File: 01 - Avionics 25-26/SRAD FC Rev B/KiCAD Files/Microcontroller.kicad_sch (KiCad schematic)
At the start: 4 parts

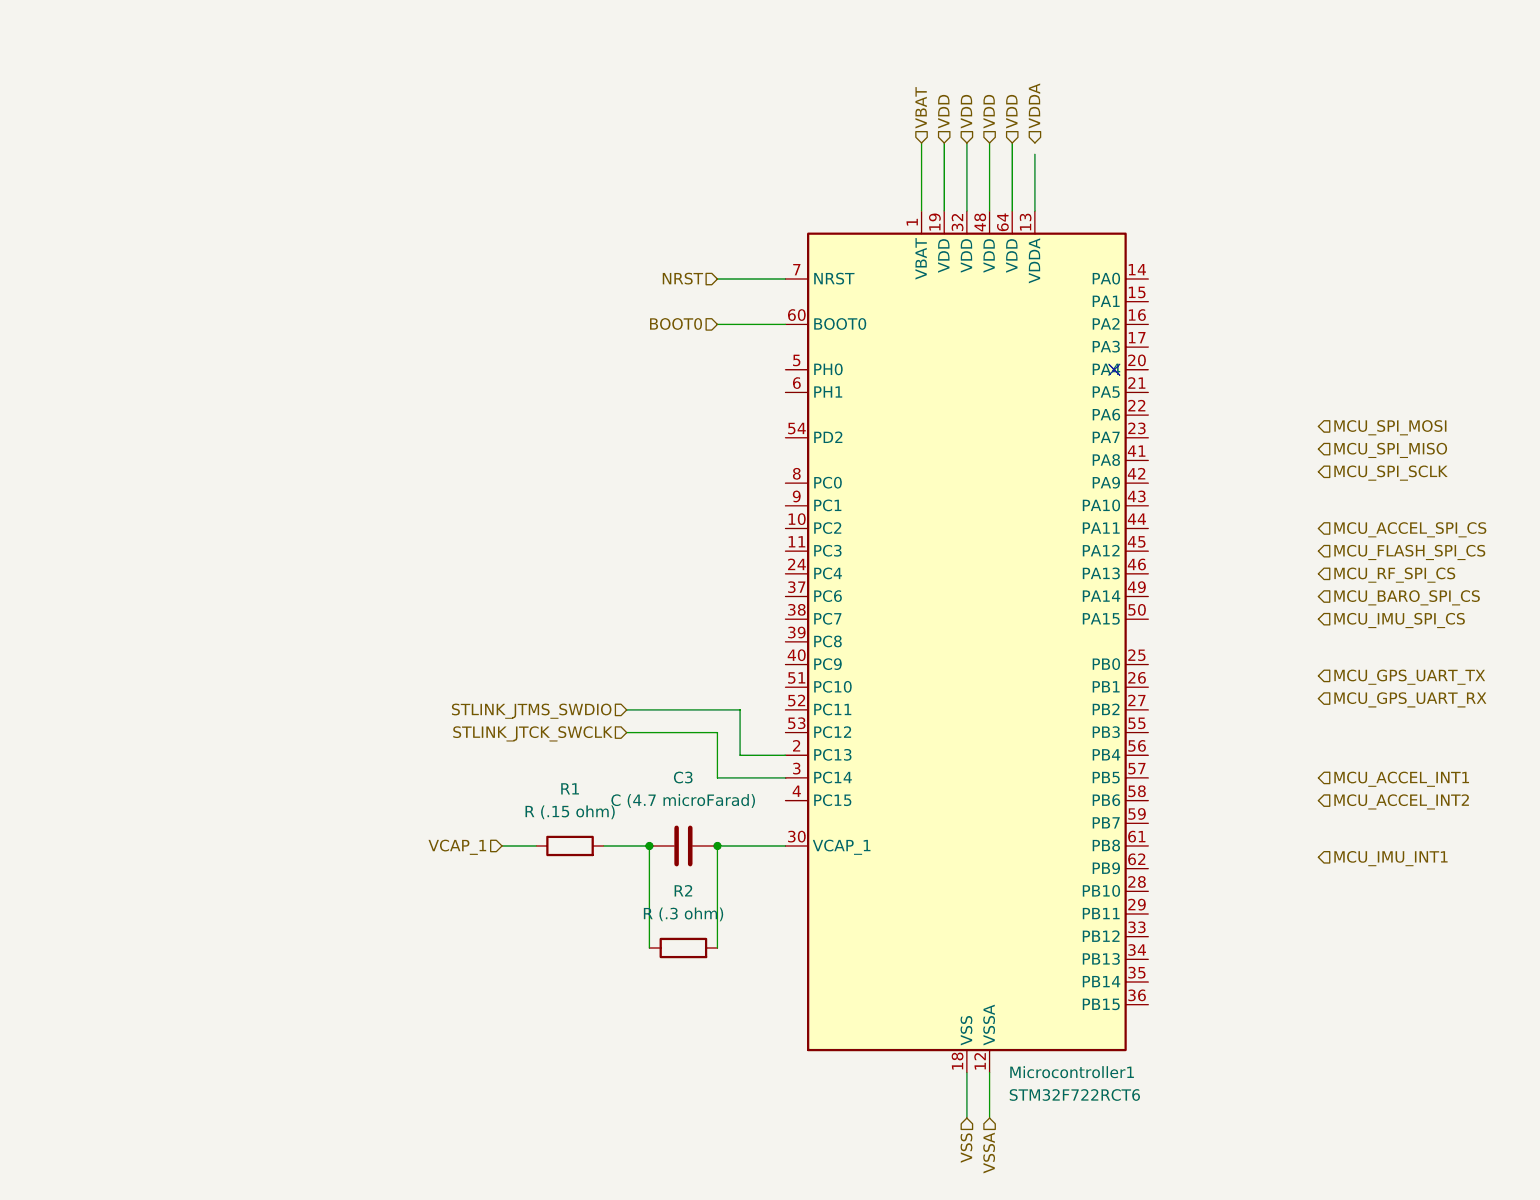
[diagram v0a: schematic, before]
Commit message: moved..... stuff
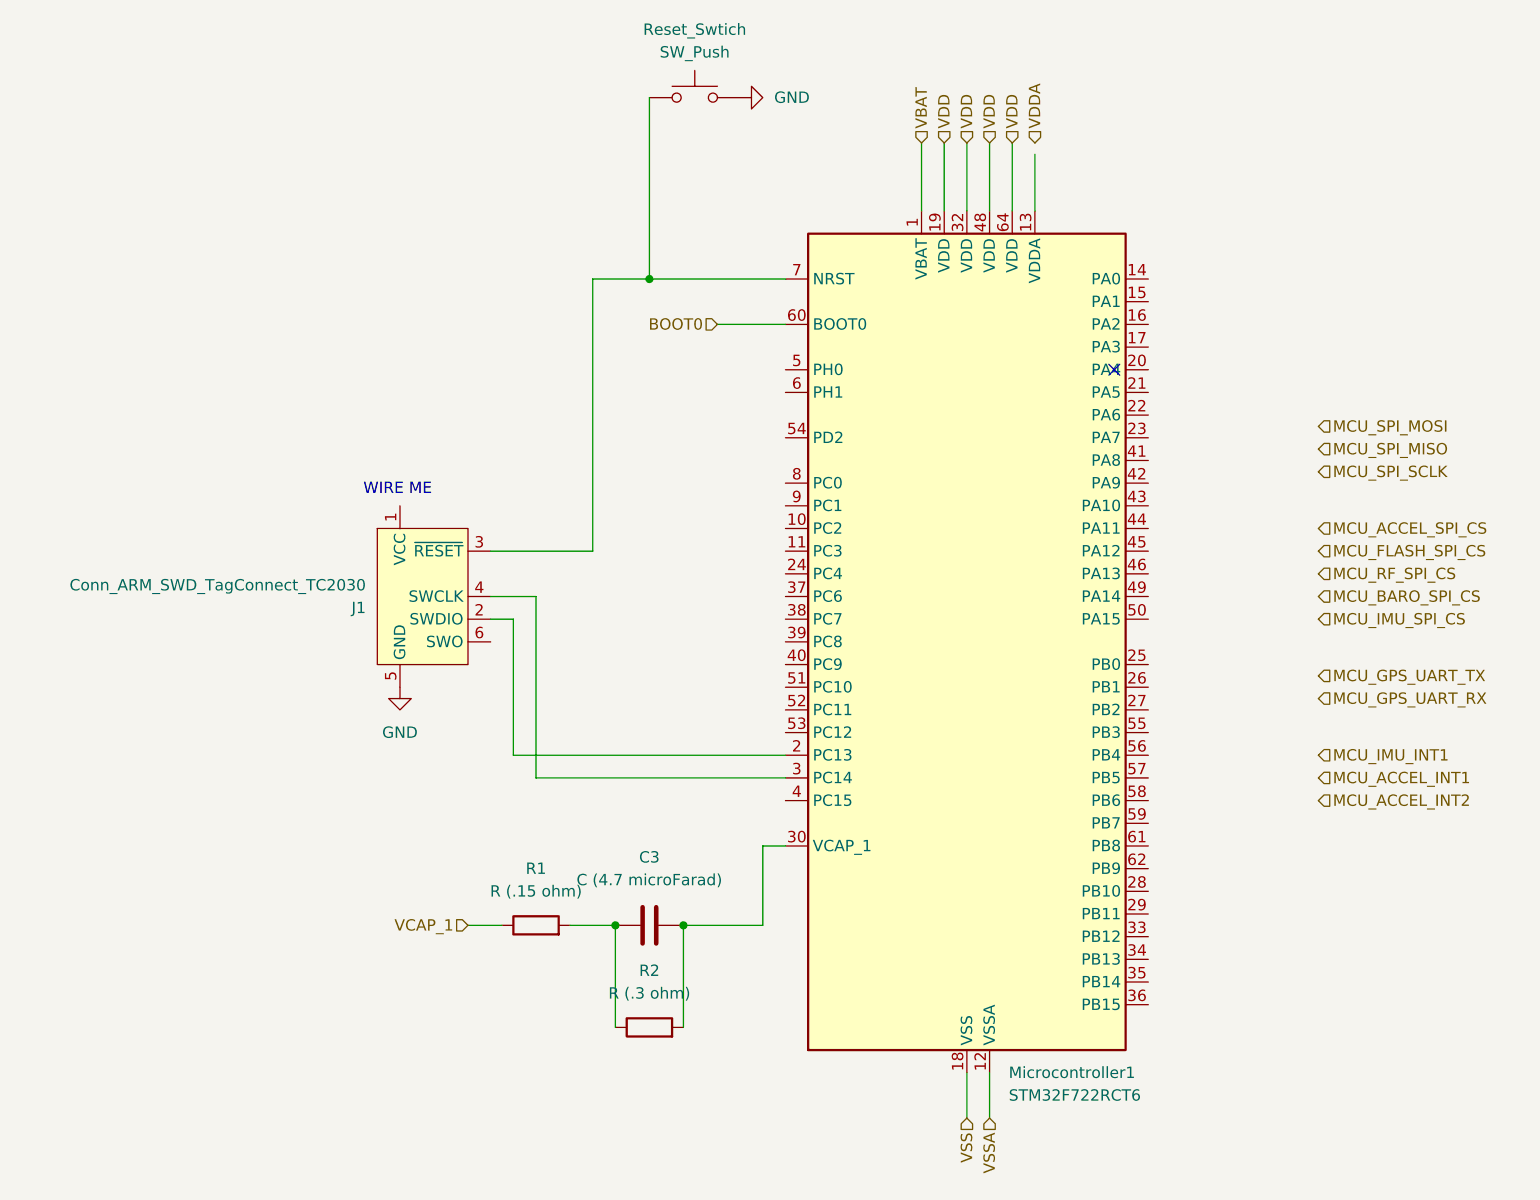
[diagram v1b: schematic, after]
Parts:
- added J1: Conn_ARM_SWD_TagConnect_TC2030, Connector:Tag-Connect_TC2030-IDC-FP_2x03_P1.27mm_Vertical, symbol Connector:Conn_ARM_SWD_TagConnect_TC2030
- added Reset_Swtich: SW_Push, symbol Switch:SW_Push
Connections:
- net NRST: no longer names the net of Microcontroller1.7 (NRST)
- net NRST: now also J1.3 (~{RESET}), Reset_Swtich.1
- net STLINK_JTCK_SWCLK: no longer names the net of Microcontroller1.3 (PC14)
- net STLINK_JTCK_SWCLK: now also J1.4 (SWCLK)
- net STLINK_JTMS_SWDIO: no longer names the net of Microcontroller1.2 (PC13)
- net STLINK_JTMS_SWDIO: now also J1.2 (SWDIO)
- new net GND: J1.5 (GND), Reset_Swtich.2
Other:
- note added: "WIRE ME"
- moved on the sheet: C3, R1, R2
